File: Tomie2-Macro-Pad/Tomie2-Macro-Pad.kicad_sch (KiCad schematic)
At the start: 24 parts, among them SW1 SW_Push, U1 ATmega32U4-A, Y1 16MHz

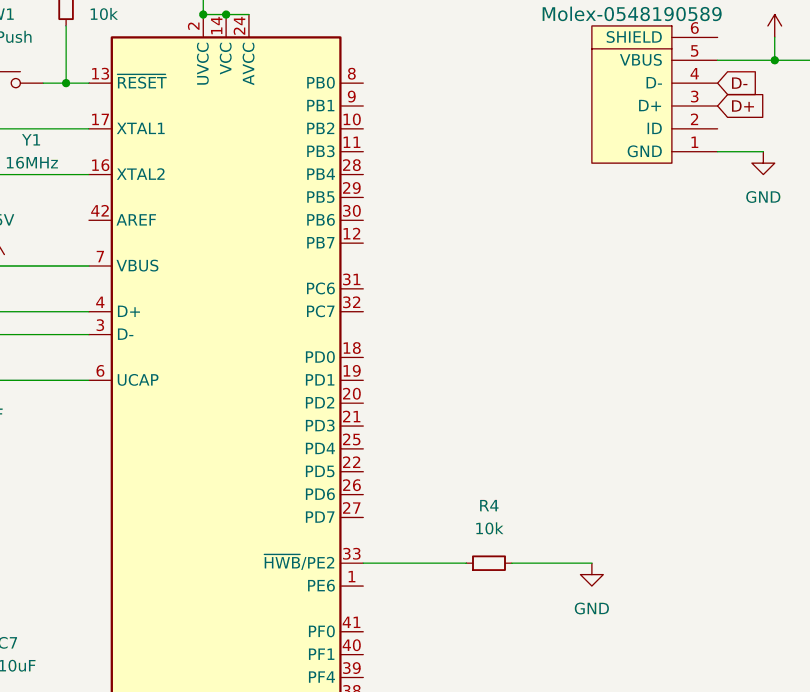
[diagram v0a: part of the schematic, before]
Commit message: PCB Finished
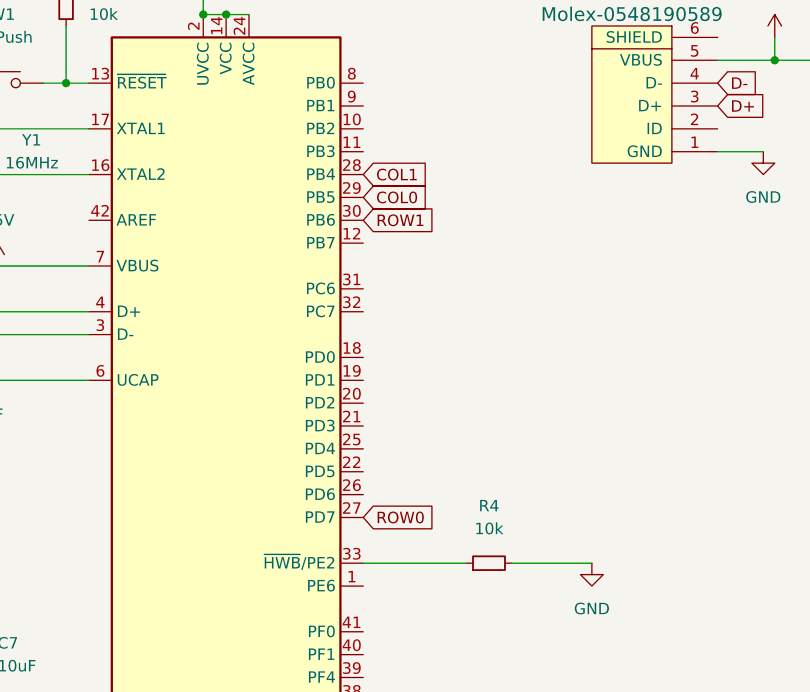
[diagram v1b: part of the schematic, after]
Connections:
- net COL0: now also U1.29 (PB5)
- net COL1: now also U1.28 (PB4)
- net ROW0: now also U1.27 (PD7)
- net ROW1: now also U1.30 (PB6)
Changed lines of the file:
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@@
+    )
+  )
+  (global_label "ROW0" (shape input) (at 114.3 116.84 0) (fields_autoplaced)
+    (effects (font (size 1.27 1.27)) (justify left))
+    (property "Intersheet References" "${INTERSHEET_REFS}" (id 0) (at 121.9745 116.7606 0)
+      (effects (font (size 1.27 1.27)) (justify left) hide)
     )
   )
@@
     (effects (font (size 1.27 1.27)) (justify left))
     (property "Intersheet References" "${INTERSHEET_REFS}" (id 0) (at 201.8506 86.7288 90)
+      (effects (font (size 1.27 1.27)) (justify left) hide)
+    )
+  )
+  (global_label "COL1" (shape input) (at 114.3 78.74 0) (fields_autoplaced)
+    (effects (font (size 1.27 1.27)) (justify left))
+    (property "Intersheet References" "${INTERSHEET_REFS}" (id 0) (at 121.5512 78.6606 0)
       (effects (font (size 1.27 1.27)) (justify left) hide)
     )
@@
     )
   )
+  (global_label "COL0" (shape input) (at 114.3 81.28 0) (fields_autoplaced)
+    (effects (font (size 1.27 1.27)) (justify left))
+    (property "Intersheet References" "${INTERSHEET_REFS}" (id 0) (at 121.5512 81.2006 0)
+      (effects (font (size 1.27 1.27)) (justify left) hide)
+    )
+  )
   (global_label "D-" (shape input) (at 153.67 68.58 0) (fields_autoplaced)
     (effects (font (size 1.27 1.27)) (justify left))
@@
       (effects (font (size 1.27 1.27)) (justify left) hide)
     )
+  )
+  (global_label "ROW1" (shape input) (at 114.3 83.82 0) (fields_autoplaced)
+    (effects (font (size 1.27 1.27)) (justify left))
+    (property "Intersheet References" "${INTERSHEET_REFS}" (id 0) (at 121.9745 83.7406 0)
+      (effects (font (size 1.27 1.27)) (justify left) hide)
+    )
